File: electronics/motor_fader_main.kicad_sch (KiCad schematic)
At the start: 30 parts, among them J1 Conn_01x04_MountingPin, J2 Program, J3 Conn_01x04_MountingPin, U1 ATtiny1616-M, U2 DRV8837

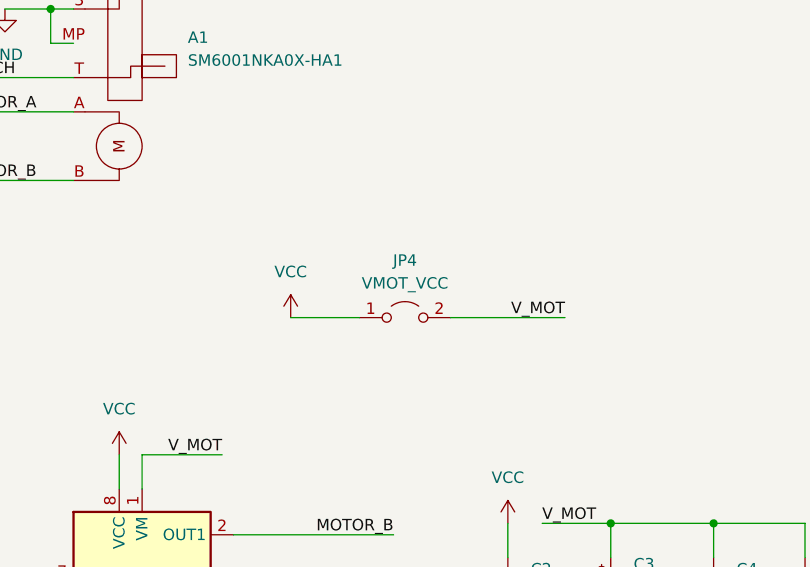
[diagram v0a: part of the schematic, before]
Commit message: minor updates, mostly ready
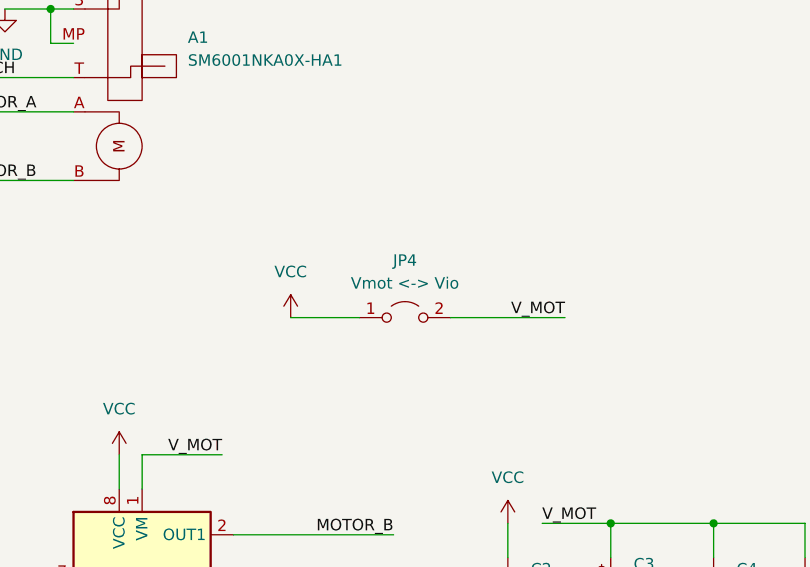
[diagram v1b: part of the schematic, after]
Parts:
- J1: footprint Connector_PinSocket_2.54mm:PinSocket_1x05_P2.54mm_Horizontal -> modified:PinSocket_1x05_P2.54mm_Horizontal_no_silk_fill
- J3: footprint Connector_PinHeader_2.54mm:PinHeader_1x05_P2.54mm_Horizontal -> modified:PinHeader_1x05_P2.54mm_Horizontal_no_pin_silk
- JP4: value VMOT_VCC -> Vmot <-> Vio; footprint modified:SolderJumper-2_P1.3mm_Open_TrianglePad1.0x1.5mm_thermal_relief -> modified:SolderJumper-2_P1.3mm_Open_TrianglePad1.0x1.5mm_thermal_relief_labelzone
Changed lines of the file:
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@@
 			)
 		)
-		(property "Footprint" "Connector_PinHeader_2.54mm:PinHeader_1x05_P2.54mm_Horizontal"
+		(property "Footprint" "modified:PinHeader_1x05_P2.54mm_Horizontal_no_pin_silk"
 			(at 82.55 181.61 0)
 			(effects
@@
 			)
 		)
-		(property "Value" "VMOT_VCC"
+		(property "Value" "Vmot <-> Vio"
 			(at 185.42 96.52 0)
 			(effects
@@
 			)
 		)
-		(property "Footprint" "modified:SolderJumper-2_P1.3mm_Open_TrianglePad1.0x1.5mm_thermal_relief"
+		(property "Footprint" "modified:SolderJumper-2_P1.3mm_Open_TrianglePad1.0x1.5mm_thermal_relief_labelzone"
 			(at 185.42 100.33 0)
 			(effects
@@
 			)
 		)
-		(property "Footprint" "Connector_PinSocket_2.54mm:PinSocket_1x05_P2.54mm_Horizontal"
+		(property "Footprint" "modified:PinSocket_1x05_P2.54mm_Horizontal_no_silk_fill"
 			(at 82.55 166.37 0)
 			(effects

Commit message: Board cleanup, BOM cleanup
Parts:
- H1, H2, J2, JP1, JP2, JP3, JP4, TP1, TP4, TP5, TP6: now left out of the parts list
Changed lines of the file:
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@@
 		(unit 1)
 		(exclude_from_sim no)
-		(in_bom yes)
+		(in_bom no)
 		(on_board yes)
 		(dnp no)
@@
 		(unit 1)
 		(exclude_from_sim no)
-		(in_bom yes)
+		(in_bom no)
 		(on_board yes)
 		(dnp no)
@@
 		(unit 1)
 		(exclude_from_sim no)
-		(in_bom yes)
+		(in_bom no)
 		(on_board yes)
 		(dnp no)
@@
 		(unit 1)
 		(exclude_from_sim no)
-		(in_bom yes)
+		(in_bom no)
 		(on_board yes)
 		(dnp no)
@@
 		(unit 1)
 		(exclude_from_sim no)
-		(in_bom yes)
+		(in_bom no)
 		(on_board yes)
 		(dnp no)
@@
 		(unit 1)
 		(exclude_from_sim no)
-		(in_bom yes)
+		(in_bom no)
 		(on_board yes)
 		(dnp no)
@@
 		(unit 1)
 		(exclude_from_sim no)
-		(in_bom yes)
+		(in_bom no)
 		(on_board yes)
 		(dnp no)
@@
 		(unit 1)
 		(exclude_from_sim no)
-		(in_bom yes)
+		(in_bom no)
 		(on_board yes)
 		(dnp no)
@@
 		(unit 1)
 		(exclude_from_sim no)
-		(in_bom yes)
+		(in_bom no)
 		(on_board yes)
 		(dnp no)
@@
 		(unit 1)
 		(exclude_from_sim no)
-		(in_bom yes)
+		(in_bom no)
 		(on_board yes)
 		(dnp no)
@@
 		(unit 1)
 		(exclude_from_sim no)
-		(in_bom yes)
+		(in_bom no)
 		(on_board yes)
 		(dnp no)
